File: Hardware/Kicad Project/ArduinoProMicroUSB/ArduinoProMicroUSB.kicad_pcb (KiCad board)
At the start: 4 copper layers, 31 x 26.4 mm, 55 parts, among them J1 Conn2, J3 FPC, Q1 MMBT3904, SW1 SW_Push, SW2 SW_Push, SW3 SW_Push, SW4 SW_Push, U1 RV-3028-C7, U3 USB-AB, U4 TPS62840DLCR, U5 ATMEGA32U4QFN, Y1 16MHz

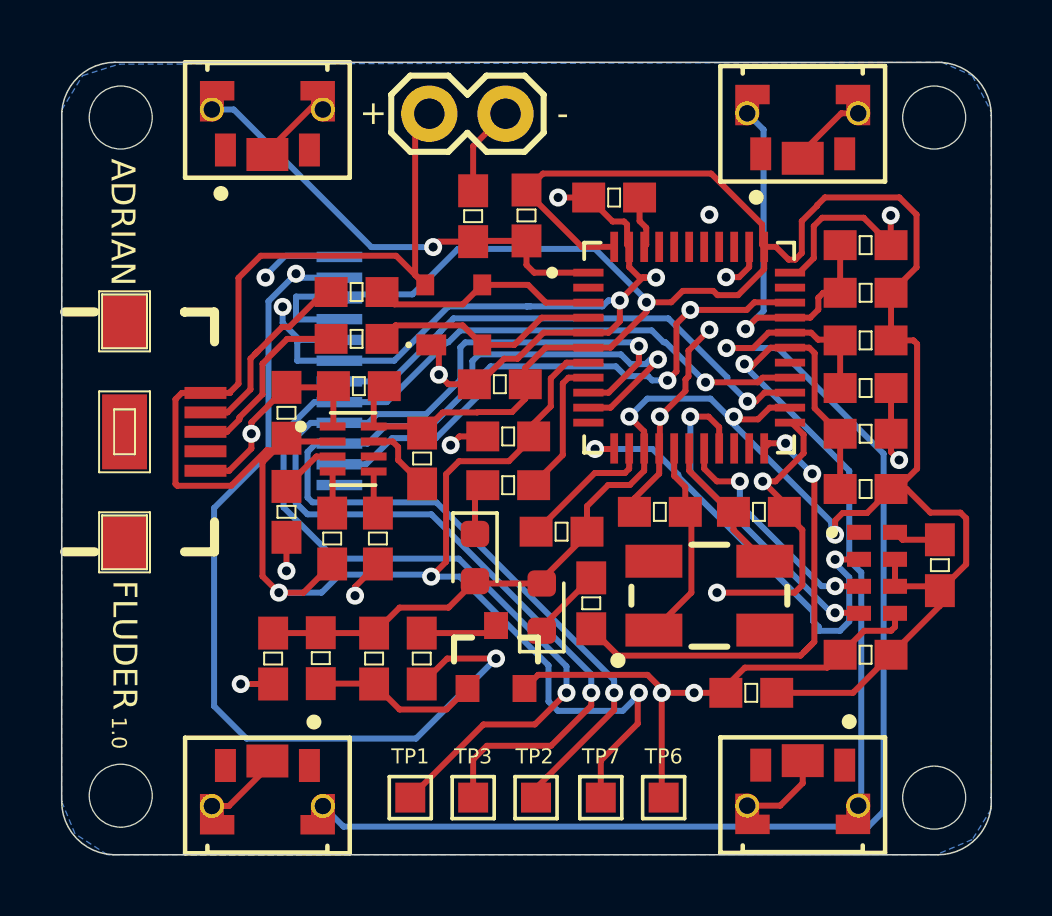
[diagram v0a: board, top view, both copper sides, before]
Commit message: checking pcb
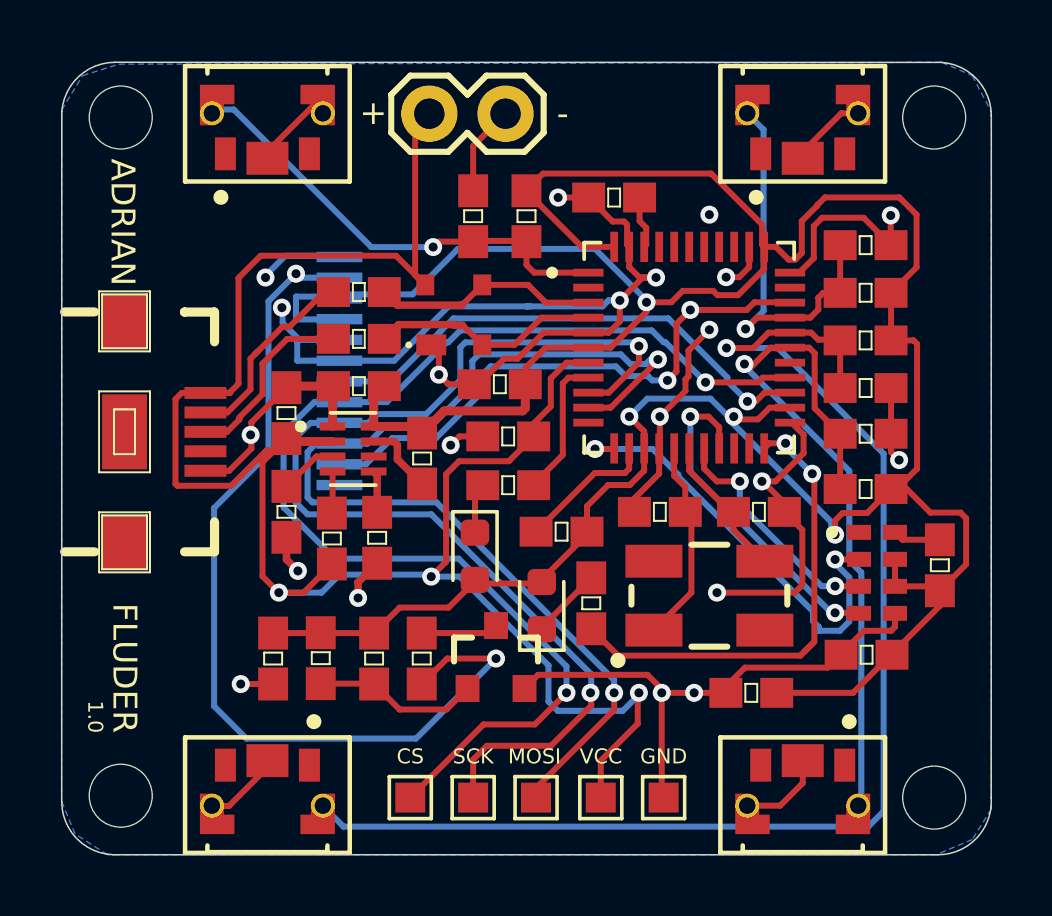
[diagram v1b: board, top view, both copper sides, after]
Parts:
- moved SW2 0.13 mm to (93.2, 72.8)
- moved R5 0.08 mm to (96.3, 78.8)
- moved R7 0.08 mm to (96.3, 80.3)
- renumbered TP1 to CS, TP6 to GND, TP2 to MOSI, TP3 to SCK, TP7 to VCC
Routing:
- net GND: track 105.1 -> 105.6 mm

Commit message: checking pcb
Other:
- copper layers 4 -> 2
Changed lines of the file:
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@@
   (layers
     (0 F.Cu signal)
-    (1 In1.Cu signal hide)
-    (2 In2.Cu signal hide)
     (31 B.Cu signal)
-    (32 B.Adhes user hide)
-    (33 F.Adhes user hide)
-    (34 B.Paste user hide)
-    (35 F.Paste user hide)
-    (36 B.SilkS user hide)
+    (32 B.Adhes user)
+    (33 F.Adhes user)
+    (34 B.Paste user)
+    (35 F.Paste user)
+    (36 B.SilkS user)
     (37 F.SilkS user)
-    (38 B.Mask user hide)
-    (39 F.Mask user hide)
-    (40 Dwgs.User user hide)
+    (38 B.Mask user)
+    (39 F.Mask user)
+    (40 Dwgs.User user)
     (41 Cmts.User user)
-    (42 Eco1.User user hide)
-    (43 Eco2.User user hide)
+    (42 Eco1.User user)
+    (43 Eco2.User user)
     (44 Edge.Cuts user)
-    (45 Margin user hide)
-    (46 B.CrtYd user hide)
+    (45 Margin user)
+    (46 B.CrtYd user)
     (47 F.CrtYd user)
     (48 B.Fab user)
-    (49 F.Fab user hide)
+    (49 F.Fab user)
   )
   (setup
